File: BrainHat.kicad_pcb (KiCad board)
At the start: 2 copper layers, 48.2 x 49.8 mm, 31 parts, among them J1 Electrodes, J2 Output, J3 Power, J4 Status, U1 AD8232, U2 TS5A3159ADBVR

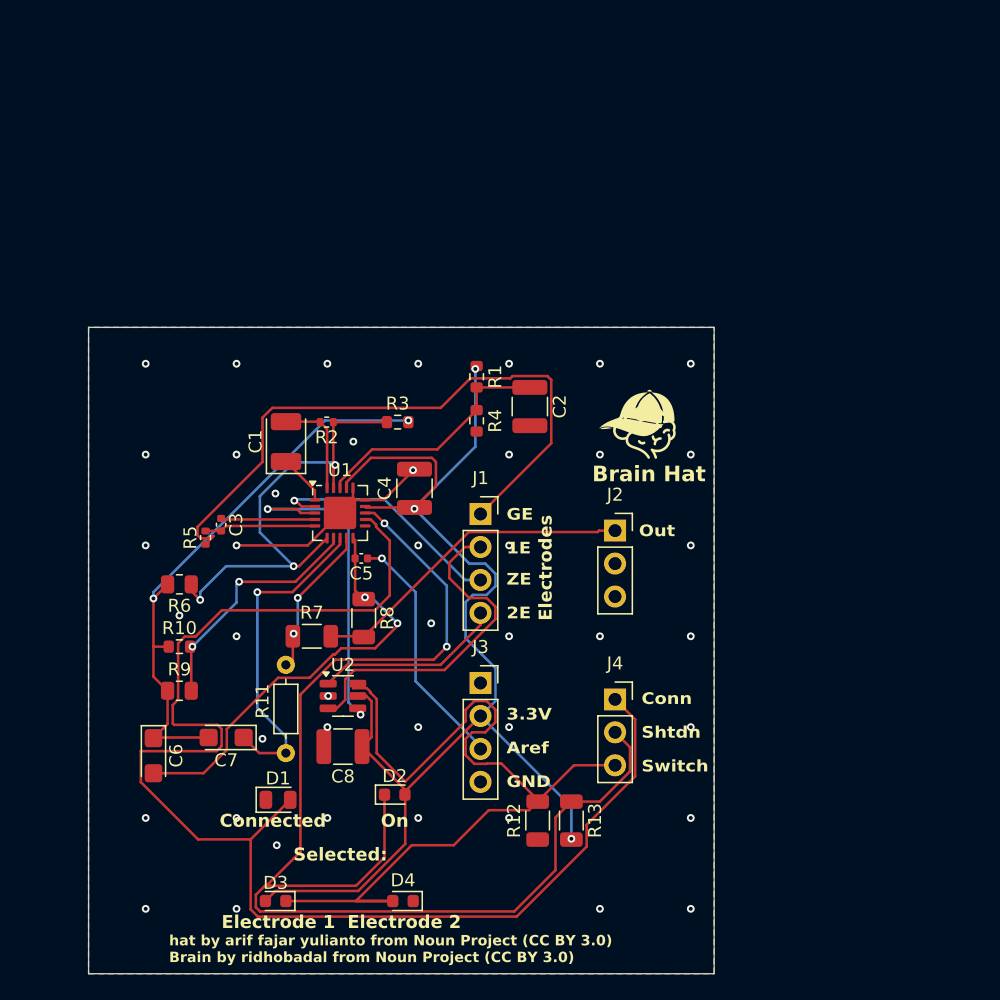
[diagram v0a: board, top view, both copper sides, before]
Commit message: YAAAA
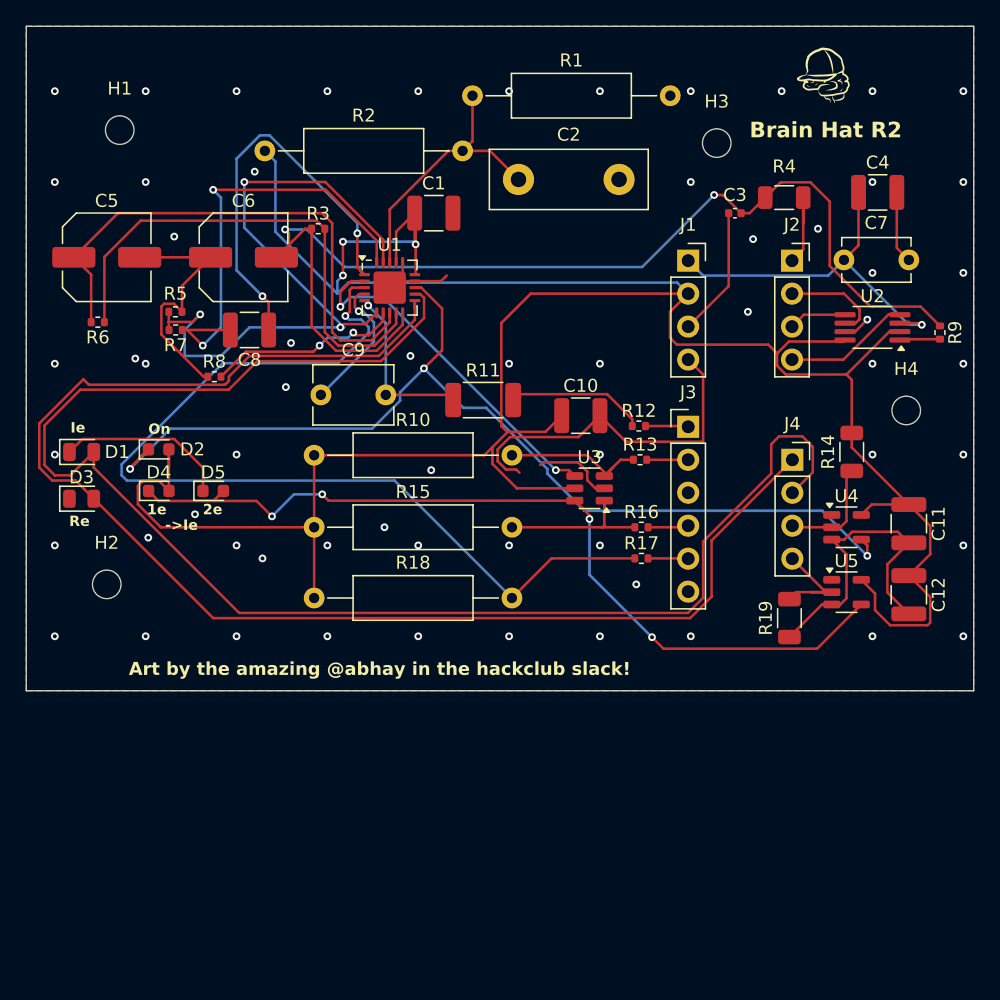
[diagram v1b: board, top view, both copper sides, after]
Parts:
- added C10: 100nF, Capacitor_SMD:C_1210_3225Metric, F.Cu at (173.5, 81.0)
- added C11: 100nF, Capacitor_SMD:C_1210_3225Metric, F.Cu at (198.8, 89.3)
- added C12: 100nF, Capacitor_SMD:C_1210_3225Metric, F.Cu at (198.8, 94.8)
- added C9: 1nF, Capacitor_THT:C_Disc_D6.0mm_W4.4mm_P5.00mm, F.Cu at (153.5, 79.4)
- added D5: XL-1608UGC-04, LED_SMD:LED_0603_1608Metric, F.Cu at (145.2, 86.8)
- added H1: MountingHole, MountingHole:MountingHole_2.2mm_M2, F.Cu at (138.0, 59.0)
- added H2: MountingHole, MountingHole:MountingHole_2.2mm_M2, F.Cu at (137.0, 94.0)
- added H3: MountingHole, MountingHole:MountingHole_2.2mm_M2, F.Cu at (184.0, 60.0)
- added H4: MountingHole, MountingHole:MountingHole_2.2mm_M2, F.Cu at (198.6, 80.6)
- added R14: 10k, Resistor_SMD:R_1206_3216Metric, F.Cu at (194.4, 83.8)
- added R15: 10M±1%, Resistor_THT:R_Axial_DIN0309_L9.0mm_D3.2mm_P15.24mm_Horizontal, F.Cu at (153.0, 89.6)
- added R16: 330k, Resistor_SMD:R_0402_1005Metric, F.Cu at (178.2, 89.6)
- added R17: 330k, Resistor_SMD:R_0402_1005Metric, F.Cu at (178.2, 92.0)
- added R18: 10M±1%, Resistor_THT:R_Axial_DIN0309_L9.0mm_D3.2mm_P15.24mm_Horizontal, F.Cu at (153.0, 95.0)
- added R19: 10k, Resistor_SMD:R_1206_3216Metric, F.Cu at (189.6, 96.6)
- added U3: TS5A3159ADBVR, Package_TO_SOT_SMD:SOT-23-6, F.Cu at (174.2, 86.6)
- added U4: SN74LV1T34DBV, Package_TO_SOT_SMD:SOT-23-5, F.Cu at (194.0, 89.6)
- added U5: SN74LV1T34DBV, Package_TO_SOT_SMD:SOT-23-5, F.Cu at (194.0, 94.6)
- C1: value CA45-B6R3K107T -> 100nF; footprint Capacitor_Tantalum_SMD:CP_EIA-3528-21_Kemet-B -> Capacitor_SMD:C_1210_3225Metric
- C2: value ECHU1C104GX5 -> 10nF; footprint Capacitor_SMD:C_1210_3225Metric -> Capacitor_THT:C_Disc_D12.0mm_W4.4mm_P7.75mm
- C3: value CC0402JRX7R9BB102 -> 14pF
- C4, C8: value ECHU1C104GX5 -> 100nF
- C5: value 0402CG140J500NT -> 220uF; footprint Capacitor_SMD:C_0402_1005Metric -> Capacitor_SMD:C_Elec_6.3x5.4
- C6: value CA45-A010K106T -> 220uF; footprint Capacitor_Tantalum_SMD:CP_EIA-3216-12_Kemet-S -> Capacitor_SMD:C_Elec_6.3x5.4
- C7: value CA45-A010K106T -> 1uF; footprint Capacitor_Tantalum_SMD:CP_EIA-3216-12_Kemet-S -> Capacitor_THT:C_Disc_D5.1mm_W3.2mm_P5.00mm
- D3: value XL-1608UGC-04 -> XL-2012UWC; footprint LED_SMD:LED_0603_1608Metric -> LED_SMD:LED_0805_2012Metric
- J1: value Electrodes -> Power
- J2, J4: footprint Connector_PinSocket_2.54mm:PinSocket_1x03_P2.54mm_Vertical -> Connector_PinSocket_2.54mm:PinSocket_1x04_P2.54mm_Vertical
- J3: value Power -> Electrodes; footprint Connector_PinSocket_2.54mm:PinSocket_1x04_P2.54mm_Vertical -> Connector_PinHeader_2.54mm:PinHeader_1x06_P2.54mm_Vertical
- R1: value ARG03BTC1002 -> 10M±1%; footprint Resistor_SMD:R_0603_1608Metric -> Resistor_THT:R_Axial_DIN0309_L9.0mm_D3.2mm_P15.24mm_Horizontal
- R10: value 0603WAD3302T5E -> 10M±1%; footprint Resistor_SMD:R_0603_1608Metric -> Resistor_THT:R_Axial_DIN0309_L9.0mm_D3.2mm_P15.24mm_Horizontal
- R11: value CF1/6W-7.5KΩ±5%T52 -> 412k; footprint Personal:R_Axial_DIN0207_L6.3mm_D2.5mm_P5.08mm_Horizontal -> Resistor_SMD:R_2010_5025Metric
- R12, R13: value 1206W4F1002T5E -> 330k; footprint Resistor_SMD:R_1206_3216Metric -> Resistor_SMD:R_0402_1005Metric
- R2: value SCR0402J330K -> 10M±1%; footprint Resistor_SMD:R_0402_1005Metric -> Resistor_THT:R_Axial_DIN0309_L9.0mm_D3.2mm_P15.24mm_Horizontal
- R3: value 0603WAD3302T5E -> 604; footprint Resistor_SMD:R_0603_1608Metric -> Resistor_SMD:R_0402_1005Metric
- R4: value ARG03BTC1002 -> 10k; footprint Resistor_SMD:R_0603_1608Metric -> Resistor_SMD:R_1206_3216Metric
- R5: value SCR0402J330K -> 1.2M
- R6: value ARG05DTC1600 -> 1k; footprint Resistor_SMD:R_0805_2012Metric -> Resistor_SMD:R_0402_1005Metric
- R7: value 1206W4F1002T5E -> 1.58M; footprint Resistor_SMD:R_1206_3216Metric -> Resistor_SMD:R_0402_1005Metric
- R8: value 1206W4F1002T5E -> 1.2M; footprint Resistor_SMD:R_1206_3216Metric -> Resistor_SMD:R_0402_1005Metric
- R9: value ARG05DTC1600 -> 330; footprint Resistor_SMD:R_0805_2012Metric -> Resistor_SMD:R_0402_1005Metric
- U2: value TS5A3159ADBVR -> ADS1251; footprint Package_TO_SOT_SMD:SOT-23-6 -> Package_SO:MSOP-8_3x3mm_P0.65mm
- moved R9 64.8 mm to (201.2, 74.6), turned to -90 degrees
- moved C7 60.2 mm to (193.8, 69.0), turned to 0 degrees
- moved U2 49.7 mm to (196.0, 74.2), turned to 180 degrees
- moved C3 46.3 mm to (185.4, 65.4), turned to 0 degrees
- moved C4 42.3 mm to (196.4, 63.8), turned to 0 degrees
- moved C6 39.0 mm to (147.5, 68.8), turned to 0 degrees
- moved D4 36.8 mm to (141.0, 86.8), turned to 0 degrees
- moved D3 34.4 mm to (135.1, 87.4), turned to 0 degrees
- moved C8 32.9 mm to (148.0, 74.4)
- moved D2 32.2 mm to (141.0, 83.6)
- moved R12 31.4 mm to (178.0, 81.8), turned to 0 degrees
- moved R11 31.2 mm to (166.0, 79.8), turned to 0 degrees
- moved D1 30.8 mm to (135.1, 83.8)
- moved C5 30.4 mm to (137.0, 68.8), turned to 0 degrees
- moved R4 29.3 mm to (189.2, 64.2), turned to 180 degrees
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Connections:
- C1 pad 1: HPDRIVE1 -> +3.3V
- C1 pad 2: HPSENSE1 -> GND
- C3 pad 1: RLDFB1 -> Aref
- C3 pad 2: RLD1 -> UFOUT1
- C4 pad 1: +3.3V -> +5V
- C5 pad 1: Aref -> REFOUT1
- C5 pad 2: UFOUT1 -> Net-(C5-Pad2)
- C6 pad 1: Net-(C6-Pad1) -> Net-(C5-Pad2)
- C7 pad 1: REFOUT1 -> +5V
- C7 pad 2: Net-(C6-Pad1) -> GND
- C8 pad 1: +3.3V -> HPDRIVE1
- C8 pad 2: GND -> HPSENSE1
- D1 pad 2: connected1 -> connectedI
- D3 pad 1: switch -> GND
- D3 pad 2: +3.3V -> connectedR
- D4 pad 1: GND -> switch
- D4 pad 2: switch -> +3.3V
- J1 pad 1: Ge -> +5V
- J1 pad 2: 1e -> +3.3V
- J1 pad 3: Ze -> Aref
- J1 pad 4: 2e -> GND
- J2 pad 2: unconnected-(J2-Pin_2-Pad2) -> SCLK
- J2 pad 3: unconnected-(J2-Pin_3-Pad3) -> DOUT/~{DRDY}
- J3 pad 1: unconnected-(J3-Pin_1-Pad1) -> Net-(J3-Pin_1)
- J3 pad 2: +3.3V -> Net-(J3-Pin_2)
- J3 pad 3: Aref -> unconnected-(J3-Pin_3-Pad3)
- J3 pad 4: GND -> Net-(J3-Pin_4)
- J4 pad 1: connected1 -> connectedR
- J4 pad 2: shutdown -> connectedI
- J4 pad 3: switch -> 5Vshutdown
- R1 pad 1: +3.3V -> Vref
- R1 pad 2: Vref -> GND
- R10 pad 1: Net-(C6-Pad1) -> +3.3V
- R10 pad 2: OPAMP+1 -> 1e
- R11 pad 1: REFOUT1 -> RLD1
- R11 pad 2: OPAMP-1 -> Ge
- R12 pad 1: GND -> Ge
- R12 pad 2: switch -> Net-(J3-Pin_1)
- R13 pad 1: shutdown -> 1e
- R13 pad 2: +3.3V -> Net-(J3-Pin_2)
- R2 pad 1: IAOUT1 -> +3.3V
- R2 pad 2: HPSENSE1 -> Vref
- R3 pad 1: IAOUT1 -> UFOUT1
- R3 pad 2: Net-(C6-Pad1) -> OPAMP-1
- R4 pad 1: Vref -> 1o
- R4 pad 2: GND -> UFOUT1
- R5 pad 1: Ge -> IAOUT1
- R5 pad 2: RLD1 -> Net-(C5-Pad2)
- R6 pad 1: IAOUT1 -> OPAMP-1
- R6 pad 2: Net-(C6-Pad1) -> REFOUT1
- R7 pad 1: OPAMP-1 -> HPSENSE1
- R7 pad 2: 1o -> IAOUT1
- R8 pad 1: UFOUT1 -> Net-(C5-Pad2)
- R8 pad 2: 1o -> OPAMP+1
- R9 pad 1: Net-(C6-Pad1) -> UFOUT1
- R9 pad 2: OPAMP+1 -> Net-(U2-IN+)
- U1 pad 11: unconnected-(U1-LOD--Pad11) -> connectedR
- U1 pad 12: connected1 -> connectedI
- U1 pad 14: +3.3V -> GND
- U1 pad 15: GND -> +3.3V
- U1 pad 2: Ze -> Ie
- U1 pad 3: Ie -> Re
- U2 pad 1: 2e -> Net-(U2-IN+)
- U2 pad 2: GND -> +3.3V
- U2 pad 3: 1e -> +5V
- U2 pad 4: Ie -> CLK
- U2 pad 5: +3.3V -> DOUT/~{DRDY}
- U2 pad 6: switch -> SCLK
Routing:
- net connectedI: track 0.00 -> 118.2 mm
- net +3.3V: track 98.4 -> 214.3 mm
- net connectedR: track 0.00 -> 108.7 mm
- net connected1: track 107.0 -> 0.00 mm
- net Re: track 0.00 -> 74.7 mm, vias 0 -> 1
- net GND: track 14.2 -> 83.9 mm, vias 43 -> 62
- net UFOUT1: track 33.0 -> 85.8 mm
- net Net-(C6-Pad1): track 44.2 -> 0.00 mm, vias 2 -> 0
- net Ge: track 49.7 -> 10.0 mm
- net +5V: track 0.00 -> 28.5 mm, vias 0 -> 1
- net HPDRIVE1: track 3.88 -> 31.7 mm, vias 0 -> 2
- net OPAMP-1: track 11.1 -> 38.9 mm, vias 2 -> 0
- net HPSENSE1: track 7.87 -> 34.1 mm, vias 0 -> 2
- net Net-(C5-Pad2): track 0.00 -> 19.6 mm
- net shutdown: track 98.1 -> 79.1 mm, vias 2 -> 3
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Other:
- board size 48.2 x 49.8 mm -> 73 x 51.2 mm
- board text added: "->Ie"
- board text added: "1e"
- board text added: "2e"
- board text added: "Art by the amazing @abhay in the hackclub slack!"
- board text added: "Brain Hat R2"
- board text added: "Ie"
- board text added: "Re"
- board text removed: "1E"
- board text removed: "2E"
- board text removed: "3.3V"
- board text removed: "Aref"
- board text removed: "Brain Hat"
- board text removed: "Conn"
- board text removed: "Connected"
- board text removed: "Electrode 1"
- board text removed: "Electrode 2"
- board text removed: "Electrodes"
- board text removed: "GE"
- board text removed: "GND"
- board text removed: "Out"
- board text removed: "Selected:"
- board text removed: "Shtdn"
- board text removed: "Switch"
- board text removed: "ZE"
- board text removed: "hat by arif fajar yulianto from Noun Project (CC BY 3.0) Brain by ridhobadal from Noun Project (CC BY 3.0)"
